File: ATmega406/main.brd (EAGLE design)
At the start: 160 x 100 mm, 9 parts, among them Q1 16M

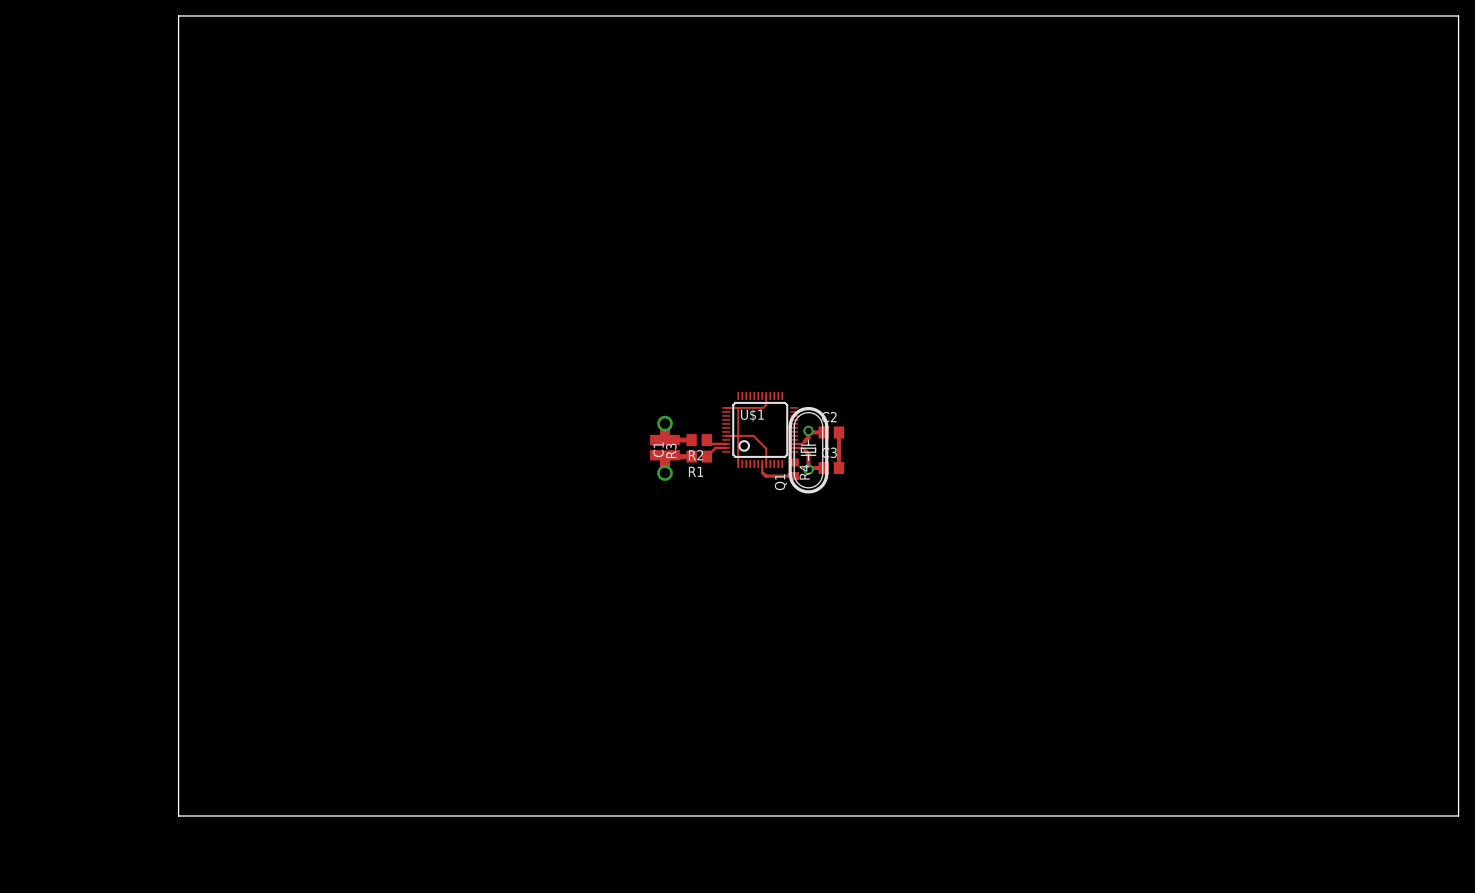
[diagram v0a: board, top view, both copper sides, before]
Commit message: afb
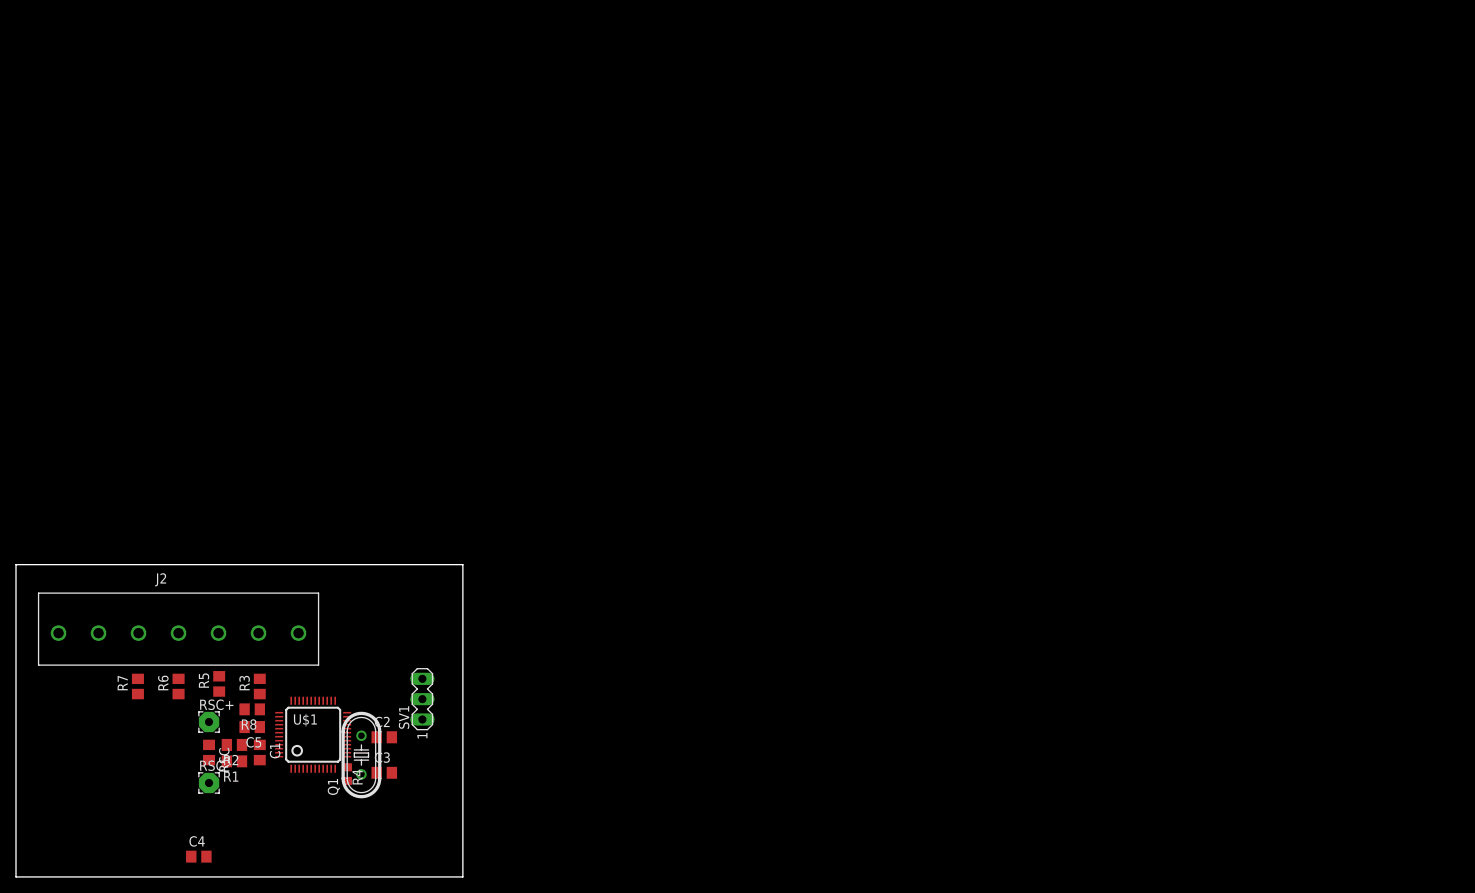
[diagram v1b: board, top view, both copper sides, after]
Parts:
- added C4, C5: 10u, rcl:C0805
- added J2: (no value), Wurth_Elektronik_Electromechanic_Terminal_Blocks_Connectors_rev17a:691136710007
- added R5, R6, R7, R8, RSC: (no value), rcl:R0805
- added RSC+, RSC-: (no value), 7_segment_lib:2,54/1,0
- added SV1: (no value), con-lstb:MA03-1
- moved R1 69.5 mm to (6.99, 6.83)
- moved R2 69.5 mm to (6.99, 8.89)
- moved R4 67.6 mm to (21.1, 5.24)
- moved C2 67.6 mm to (25.7, 9.84)
- moved C3 67.6 mm to (25.7, 5.40)
- moved Q1 67.6 mm to (22.9, 7.62)
- moved U$1 67.6 mm to (16.8, 10.2)
- moved C1 64.3 mm to (10.2, 7.94), turned to 270 degrees
- moved R3 57.8 mm to (10.2, 16.2), turned to 90 degrees
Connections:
- net N$9 renamed VCC
- new net BAT+: J2.6, R3.2
- new net BAT-: J2.2, R2.2, R8.2, RSC+.1, RSC.1
- new net BAT1: J2.3, R7.2
- new net BAT2: J2.4, R6.2
- new net BAT3: J2.5, R5.2
- new net GND: C2.2, C3.2, C4.2, C5.2, J2.1, R1.2, RSC-.1, RSC.2, SV1.3, U$1.1, U$1.16, U$1.29, U$1.37, U$1.44, U$1.8
- new net N$10: R6.1, U$1.40
- new net N$11: R7.1, U$1.41
- new net N$12: R8.1, U$1.42
- new net N$9: C5.1, U$1.43
- new net SCL: SV1.1, U$1.23
- new net SDA: SV1.2, U$1.24
- new net VIN: J2.7, U$1.34
- net N$1: now also C4.1, U$1.6; no longer C2.2, C3.2, U$1.1, U$1.16, U$1.29, U$1.37, U$1.44, U$1.8
- net N$2: now also C1.1
- net N$3: now also U$1.38; no longer C1.2, R2.2
- net N$4: now also R5.1, U$1.39; no longer C1.1, R1.2, R3.2
- net N$5: now also C1.2
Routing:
- net N$1: track 25.4 -> 0.00 mm
- net N$4: track 6.74 -> 0.00 mm, vias 1 -> 0
- net N$3: track 6.51 -> 0.00 mm, vias 1 -> 0
- net N$7: track 6.02 -> 0.00 mm
- net VCC: track 5.30 -> 0.00 mm
- net N$6: track 4.92 -> 0.00 mm
- net N$5: track 2.87 -> 0.00 mm
- net N$2: track 2.62 -> 0.00 mm
- net N$8: track 1.34 -> 0.00 mm
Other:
- board size 160 x 100 mm -> 55.9 x 39 mm
